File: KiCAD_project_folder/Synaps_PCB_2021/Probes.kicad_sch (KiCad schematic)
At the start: 3 parts, among them J3 Conn_02x10_MountingPin

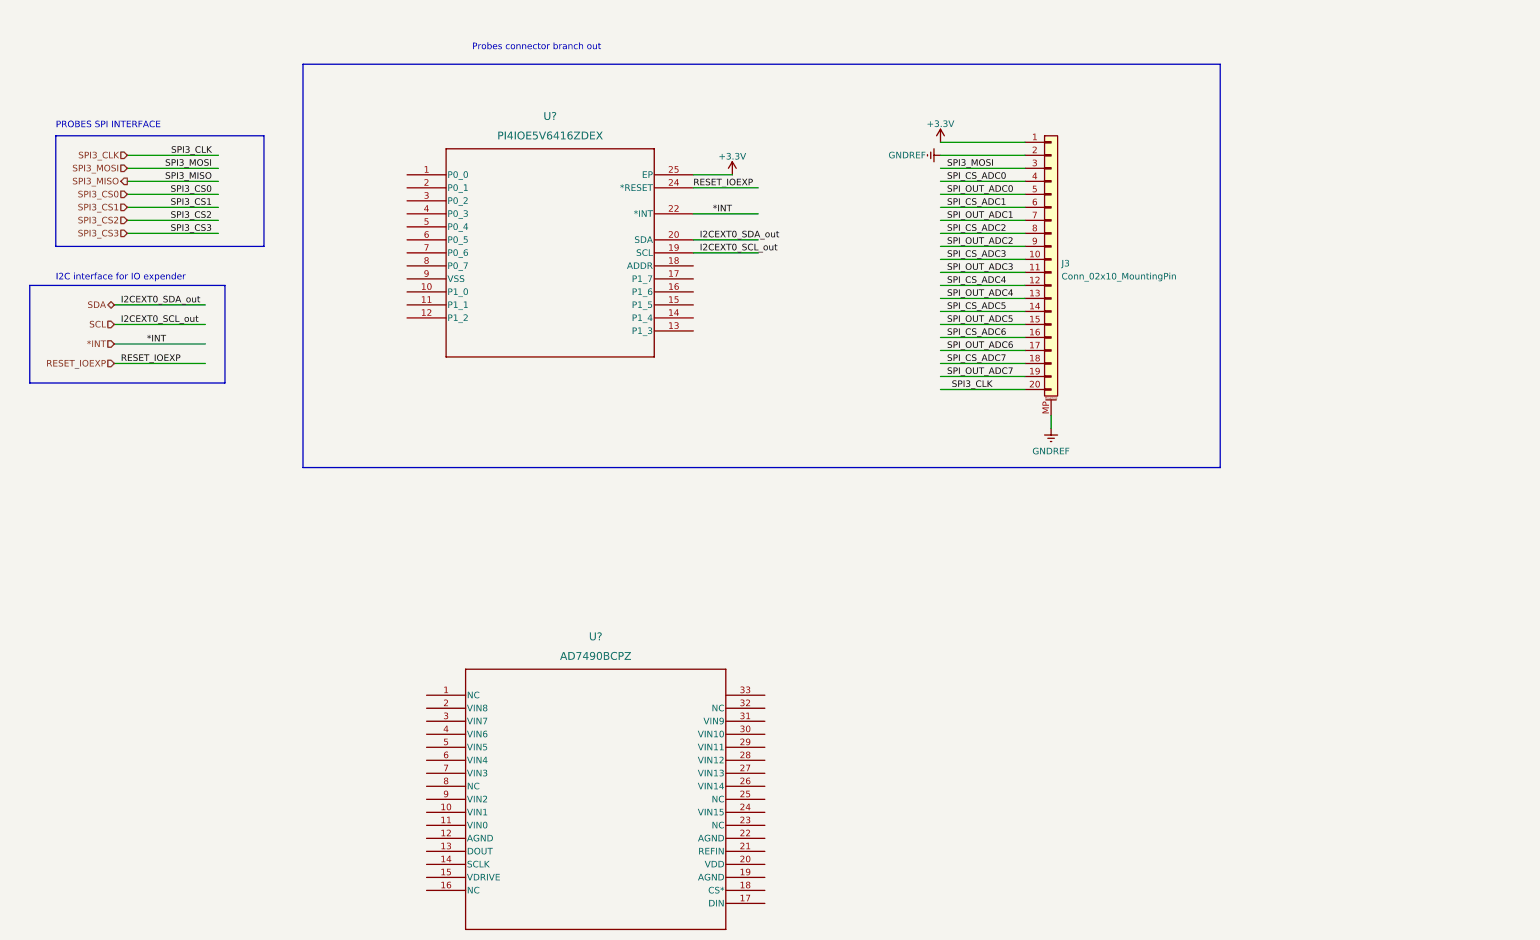
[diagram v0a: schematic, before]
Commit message: schematic finished
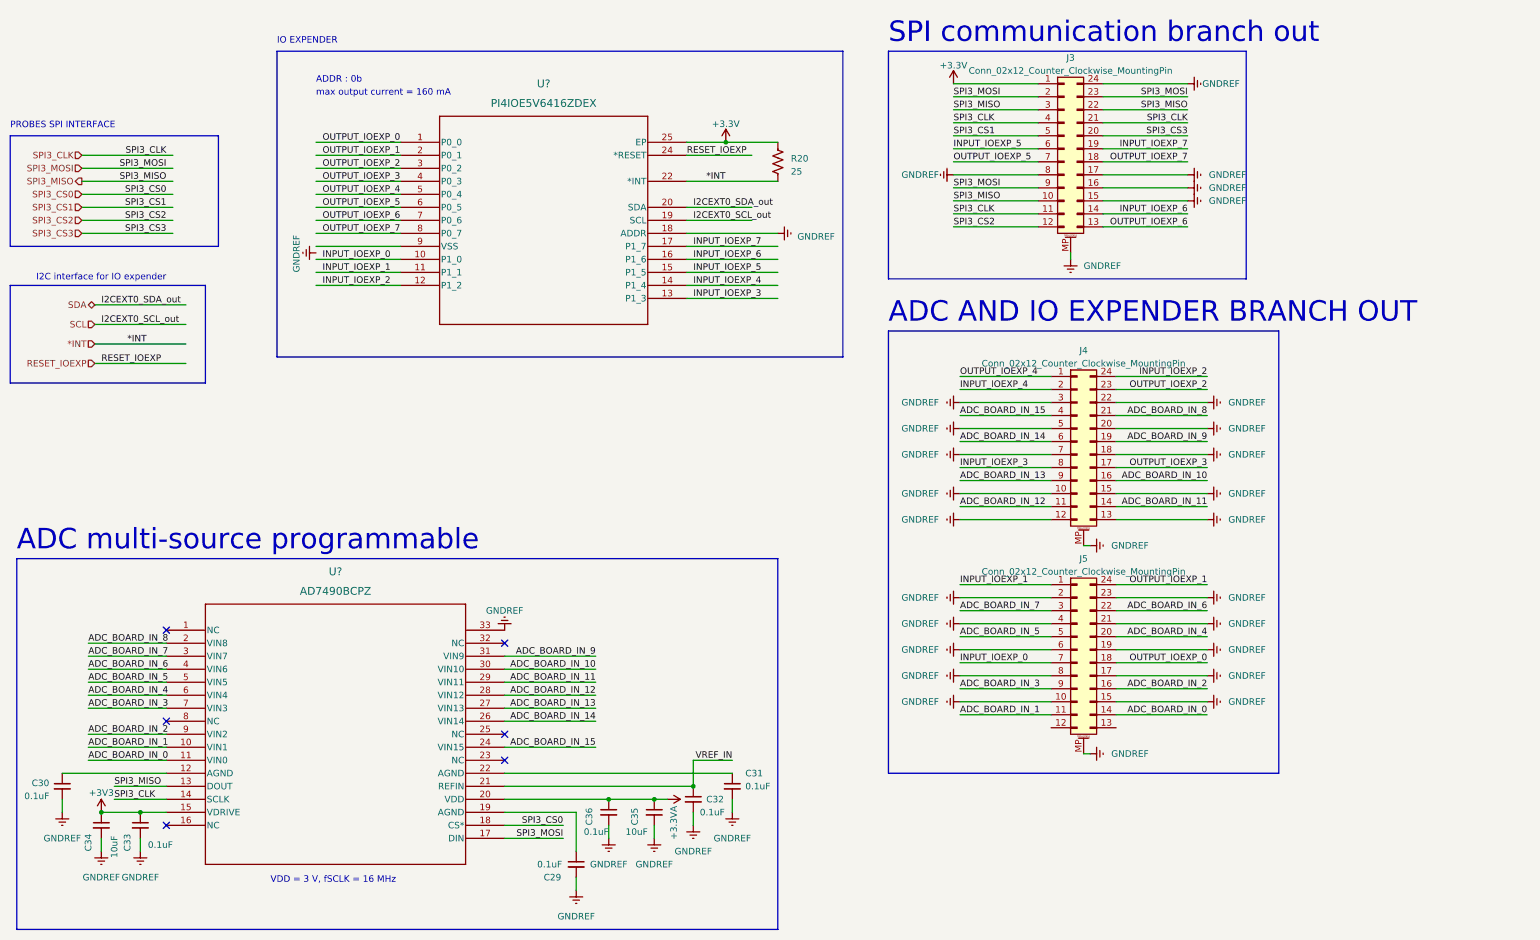
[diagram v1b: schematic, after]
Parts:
- removed J3: Conn_02x10_MountingPin, Connector_PinHeader_2.54mm:PinHeader_2x10_P2.54mm_Vertical_SMD, symbol Connector_Generic_MountingPin:Conn_01x20_MountingPin
- added C29, C30, C31, C32, C33, C36: 0.1uF, symbol Device:C_Small
- added C34, C35: 10uF, symbol Device:C_Small
- added J3, J4, J5: Conn_02x12_Counter_Clockwise_MountingPin, symbol Connector_Generic_MountingPin:Conn_02x12_Counter_Clockwise_MountingPin
- added R20: 25, symbol Device:R_US
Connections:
- net *INT: now also R20.2
- net +3V3: now also U?.15 (VDRIVE), C33.1, C34.1, J3.1 (Pin_1), R20.1
- net GNDREF: now also U?.18 (ADDR), U?.33, C29.2, C30.2, C31.2, C32.2, C33.2, C34.2, C35.2, C36.2, J3.15 (Pin_15), J3.16 (Pin_16), J3.17 (Pin_17), J3.24 (Pin_24), J3.8 (Pin_8), J3.MP (MountPin), J4.10 (Pin_10), J4.12 (Pin_12), J4.13 (Pin_13), J4.15 (Pin_15), J4.18 (Pin_18), J4.20 (Pin_20), J4.22 (Pin_22), J4.3 (Pin_3), J4.5 (Pin_5), J4.7 (Pin_7), J4.MP (MountPin), J5.10 (Pin_10), J5.15 (Pin_15), J5.17 (Pin_17), J5.19 (Pin_19), J5.2 (Pin_2), J5.21 (Pin_21), J5.23 (Pin_23), J5.4 (Pin_4), J5.6 (Pin_6), J5.8 (Pin_8), J5.MP (MountPin)
- net SPI3_CLK: now also U?.14 (SCLK), J3.11 (Pin_11), J3.21 (Pin_21), J3.4 (Pin_4)
- net SPI3_CS0: now also U?.18 (CS*)
- net SPI3_CS1: now also J3.5 (Pin_5)
- net SPI3_CS2: now also J3.12 (Pin_12)
- net SPI3_CS3: now also J3.20 (Pin_20)
- net SPI3_MISO: now also U?.13 (DOUT), J3.10 (Pin_10), J3.22 (Pin_22), J3.3 (Pin_3)
- net SPI3_MOSI: now also U?.17 (DIN), J3.2 (Pin_2), J3.23 (Pin_23), J3.9 (Pin_9)
- net OUTPUT_IOEXP_0: now reaches U?.1 (P0_0)
- net OUTPUT_IOEXP_0: now also J5.18 (Pin_18)
- net INPUT_IOEXP_0: now reaches U?.10 (P1_0)
- net INPUT_IOEXP_0: now also J5.7 (Pin_7)
- net INPUT_IOEXP_1: now reaches U?.11 (P1_1)
- net INPUT_IOEXP_1: now also J5.1 (Pin_1)
- net INPUT_IOEXP_2: now reaches U?.12 (P1_2)
- net INPUT_IOEXP_2: now also J4.24 (Pin_24)
- net INPUT_IOEXP_3: now reaches U?.13 (P1_3)
- net INPUT_IOEXP_3: now also J4.8 (Pin_8)
- net INPUT_IOEXP_4: now reaches U?.14 (P1_4)
- net INPUT_IOEXP_4: now also J4.2 (Pin_2)
- net INPUT_IOEXP_5: now reaches U?.15 (P1_5)
- net INPUT_IOEXP_5: now also J3.6 (Pin_6)
- net INPUT_IOEXP_6: now reaches U?.16 (P1_6)
- net INPUT_IOEXP_6: now also J3.14 (Pin_14)
- net INPUT_IOEXP_7: now reaches U?.17 (P1_7)
- net INPUT_IOEXP_7: now also J3.19 (Pin_19)
- net OUTPUT_IOEXP_1: now reaches U?.2 (P0_1)
- net OUTPUT_IOEXP_1: now also J5.24 (Pin_24)
- net OUTPUT_IOEXP_2: now reaches U?.3 (P0_2)
- net OUTPUT_IOEXP_2: now also J4.23 (Pin_23)
- net OUTPUT_IOEXP_3: now reaches U?.4 (P0_3)
- net OUTPUT_IOEXP_3: now also J4.17 (Pin_17)
- net OUTPUT_IOEXP_4: now reaches U?.5 (P0_4)
- net OUTPUT_IOEXP_4: now also J4.1 (Pin_1)
- net OUTPUT_IOEXP_5: now reaches U?.6 (P0_5)
- net OUTPUT_IOEXP_5: now also J3.7 (Pin_7)
- net OUTPUT_IOEXP_6: now reaches U?.7 (P0_6)
- net OUTPUT_IOEXP_6: now also J3.13 (Pin_13)
- net OUTPUT_IOEXP_7: now reaches U?.8 (P0_7)
- net OUTPUT_IOEXP_7: now also J3.18 (Pin_18)
- net ADC_BOARD_IN_1: now reaches U?.10 (VIN1)
- net ADC_BOARD_IN_1: now also J5.11 (Pin_11)
- net ADC_BOARD_IN_0: now reaches U?.11 (VIN0)
- net ADC_BOARD_IN_0: now also J5.14 (Pin_14)
- net at U?.12 (AGND): now also C30.1
- net at U?.19 (AGND): now also C29.1
- net ADC_BOARD_IN_8: now reaches U?.2 (VIN8)
- net ADC_BOARD_IN_8: now also J4.21 (Pin_21)
- net +3.3VA: now reaches U?.20 (VDD)
- net +3.3VA: now also C35.1, C36.1
- net VREF_IN: now reaches U?.21 (REFIN)
- net VREF_IN: now also C32.1
- net at U?.22 (AGND): now also C31.1
- net ADC_BOARD_IN_15: now reaches U?.24 (VIN15)
- net ADC_BOARD_IN_15: now also J4.4 (Pin_4)
- net ADC_BOARD_IN_14: now reaches U?.26 (VIN14)
- net ADC_BOARD_IN_14: now also J4.6 (Pin_6)
- net ADC_BOARD_IN_13: now reaches U?.27 (VIN13)
- net ADC_BOARD_IN_13: now also J4.9 (Pin_9)
- net ADC_BOARD_IN_12: now reaches U?.28 (VIN12)
- net ADC_BOARD_IN_12: now also J4.11 (Pin_11)
- net ADC_BOARD_IN_11: now reaches U?.29 (VIN11)
- net ADC_BOARD_IN_11: now also J4.14 (Pin_14)
- net ADC_BOARD_IN_7: now reaches U?.3 (VIN7)
- net ADC_BOARD_IN_7: now also J5.3 (Pin_3)
- net ADC_BOARD_IN_10: now reaches U?.30 (VIN10)
- net ADC_BOARD_IN_10: now also J4.16 (Pin_16)
- net ADC_BOARD_IN_9: now reaches U?.31 (VIN9)
- net ADC_BOARD_IN_9: now also J4.19 (Pin_19)
- net ADC_BOARD_IN_6: now reaches U?.4 (VIN6)
- net ADC_BOARD_IN_6: now also J5.22 (Pin_22)
- net ADC_BOARD_IN_5: now reaches U?.5 (VIN5)
- net ADC_BOARD_IN_5: now also J5.5 (Pin_5)
- net ADC_BOARD_IN_4: now reaches U?.6 (VIN4)
- net ADC_BOARD_IN_4: now also J5.20 (Pin_20)
- net ADC_BOARD_IN_3: now reaches U?.7 (VIN3)
- net ADC_BOARD_IN_3: now also J5.9 (Pin_9)
- net ADC_BOARD_IN_2: now reaches U?.9 (VIN2)
- net ADC_BOARD_IN_2: now also J5.16 (Pin_16)
- no-connect marks 0 -> 6
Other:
- note added: "ADC AND IO EXPENDER BRANCH OUT"
- note added: "ADC multi-source programmable"
- note added: "ADDR : 0b"
- note added: "IO EXPENDER"
- note added: "SPI communication branch out"
- note added: "VDD = 3 V, fSCLK = 16 MHz"
- note added: "max output current = 160 mA"
- note removed: "Probes connector branch out"
- moved on the sheet: U?
